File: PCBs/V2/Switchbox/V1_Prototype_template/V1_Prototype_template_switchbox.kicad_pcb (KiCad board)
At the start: 2 copper layers, 48 x 28 mm, 11 parts, among them J1 Conn_02x10_Top_Bottom, J2 Conn_02x10_Top_Bottom, J3 Conn_02x10_Top_Bottom, J3(IN)1 01x04 magnetic connector, J5(OUT)1 01x04 magnetic connector

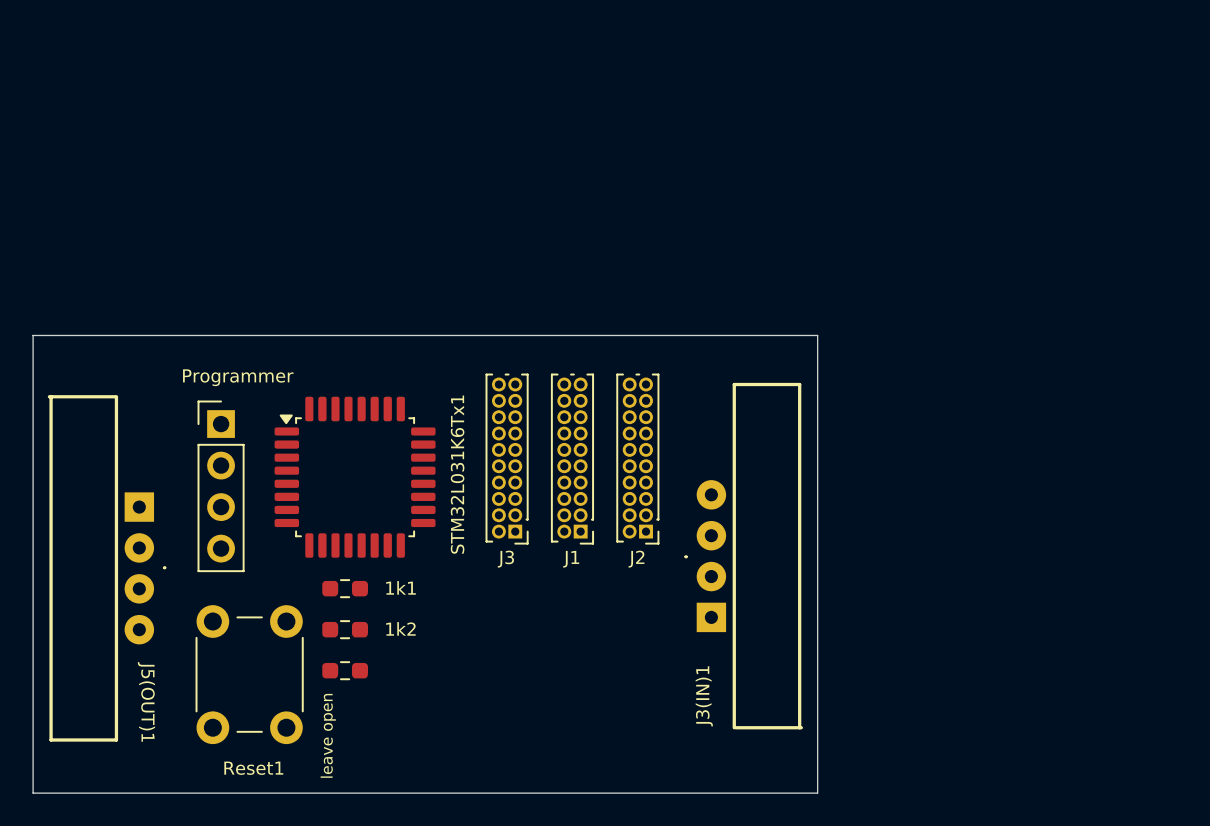
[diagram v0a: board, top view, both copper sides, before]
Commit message: PCB For switchbox prototype done
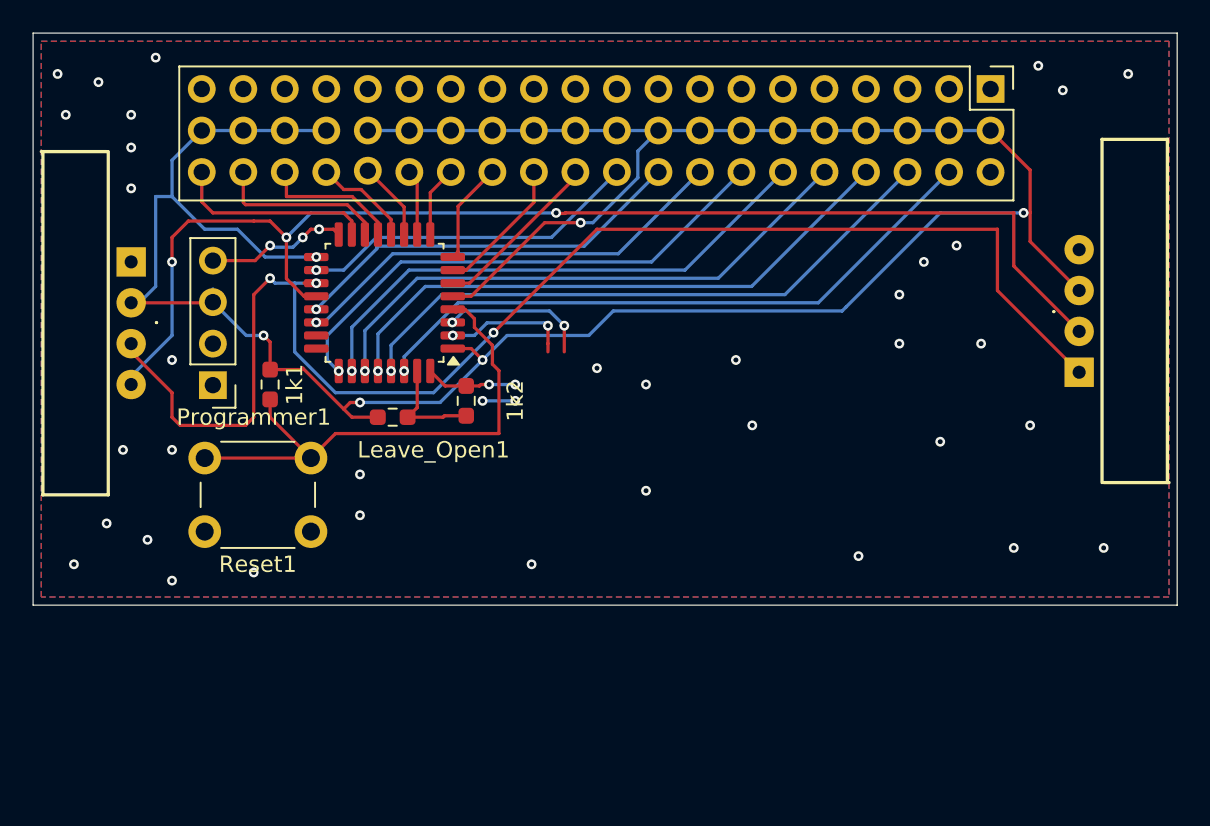
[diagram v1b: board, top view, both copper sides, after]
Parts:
- removed J1, J2, J3: Conn_02x10_Top_Bottom, Connector_PinHeader_1.00mm:PinHeader_2x10_P1.00mm_Vertical
- removed Programmer: Conn_01x04, Connector_PinHeader_2.54mm:PinHeader_1x04_P2.54mm_Vertical
- removed leave open: R, Resistor_SMD:R_0603_1608Metric_Pad0.98x0.95mm_HandSolder
- added Leave_Open1: R, Resistor_SMD:R_0603_1608Metric_Pad0.98x0.95mm_HandSolder, F.Cu at (94.0, 82.5)
- added Programmer1: Conn_01x04, Connector_PinHeader_2.54mm:PinHeader_1x04_P2.54mm_Vertical, F.Cu at (83.0, 80.5)
- added U1: ~, FootprintLibrary:PinHeader_03x20, F.Cu at (130.6, 62.4)
- moved J5(OUT)1 63.5 mm to (138.0, 76.0), turned to 90 degrees
- moved J3(IN)1 42.0 mm to (76.0, 76.8), turned to -90 degrees
- moved 1k2 15.8 mm to (98.5, 81.5), turned to 90 degrees
- moved 1k1 13.3 mm to (86.5, 80.5), turned to -90 degrees
- moved STM32L031K6Tx1 10.8 mm to (93.5, 75.5), turned to 180 degrees
- moved Reset1 5.70 mm to (89.0, 89.5), turned to 180 degrees
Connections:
- J5(OUT)1 pad 1: /GND -> /UART_TX(PA9)
- J5(OUT)1 pad 2: /VCC -> /UART_RX(PA10)
- J5(OUT)1 pad 3: /UART_RX(PA10) -> /VCC
- J5(OUT)1 pad 4: /UART_TX(PA9) -> /GND
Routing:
- net /VCC: track 0.00 -> 169.3 mm, vias 0 -> 6
- net /UART_TX(PA9): track 0.00 -> 87.0 mm, vias 0 -> 3
- net /UART_RX(PA10): track 0.00 -> 76.9 mm, vias 0 -> 3
- net /PB7: track 0.00 -> 38.9 mm, vias 0 -> 1
- net /PB6: track 0.00 -> 37.6 mm, vias 0 -> 1
- net /PB5: track 0.00 -> 36.2 mm, vias 0 -> 1
- net /PB4: track 0.00 -> 34.6 mm, vias 0 -> 1
- net /PB3: track 0.00 -> 33.0 mm, vias 0 -> 1
- net Net-(STM32L031K6Tx1-NRST): track 0.00 -> 32.7 mm
- net /PA15: track 0.00 -> 32.0 mm, vias 0 -> 1
- net /PA12: track 0.00 -> 27.3 mm, vias 0 -> 1
- net /PA11: track 0.00 -> 24.5 mm, vias 0 -> 1
- net /PA8: track 0.00 -> 20.9 mm, vias 0 -> 1
- net /GND: track 0.00 -> 16.6 mm, vias 0 -> 43
- net /PB1: track 0.00 -> 12.3 mm
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- added copper zone on B.Cu, net /GND
- added copper zone on F.Cu, net /GND
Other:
- board size 48 x 28 mm -> 70 x 35 mm
